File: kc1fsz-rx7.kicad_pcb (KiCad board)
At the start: 2 copper layers, 35.8 x 29.5 mm, 18 parts, among them J1 IQ, J2 Power, J3 Config, J4 Conn_01x06, U1 PCM1804DBR

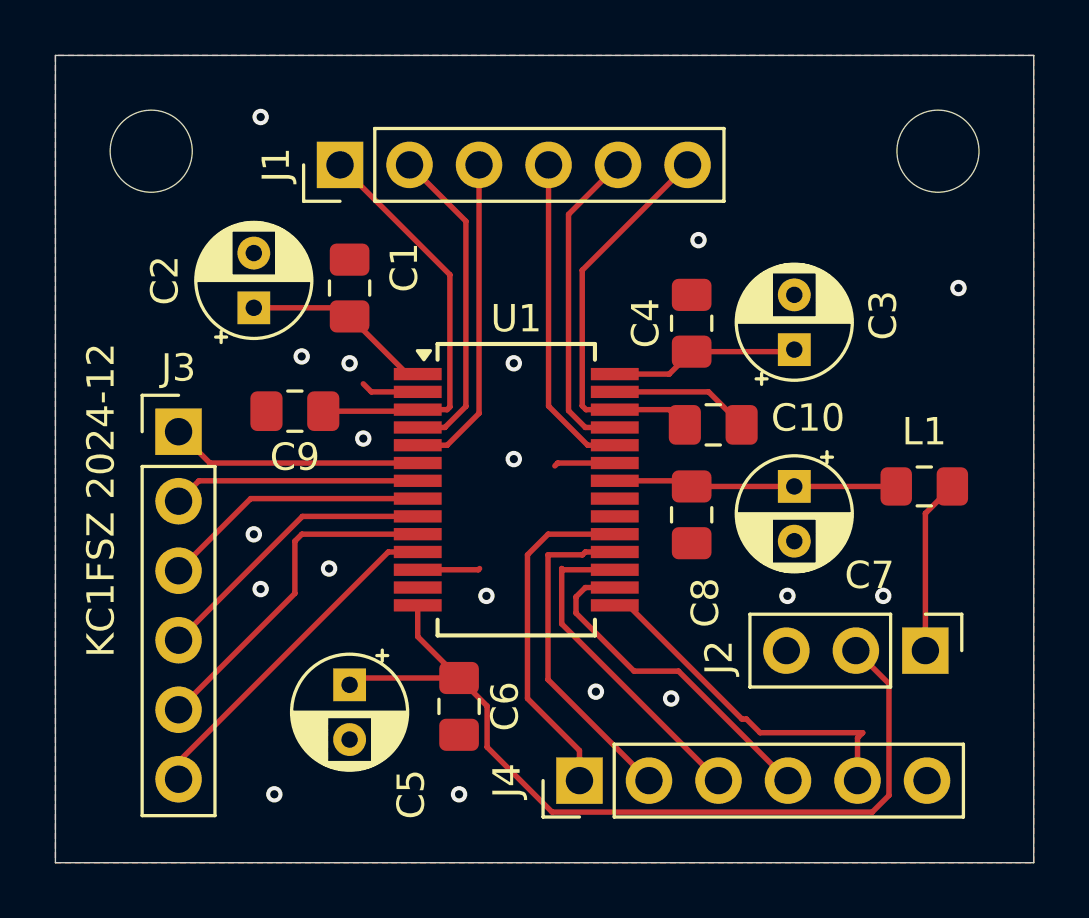
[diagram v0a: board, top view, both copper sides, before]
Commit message: Final board being sent to OSHPARK
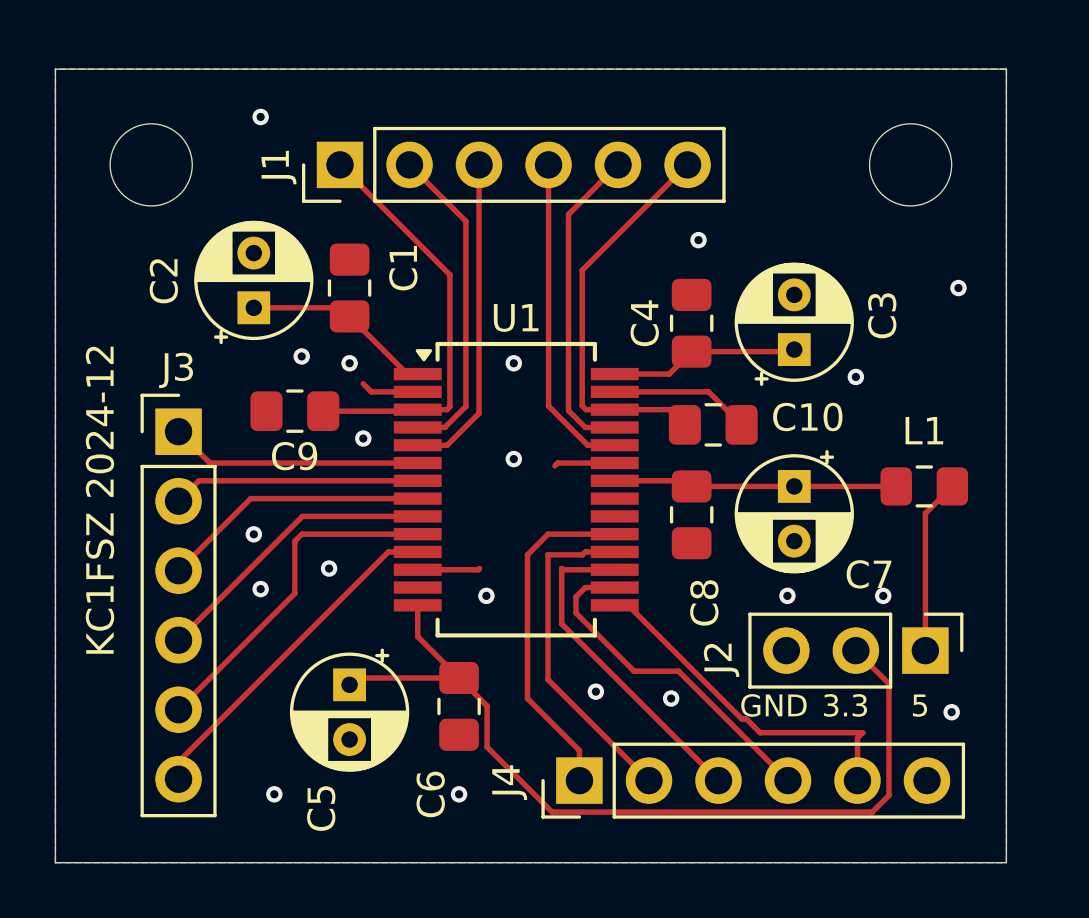
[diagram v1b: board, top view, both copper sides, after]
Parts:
- moved H2 1.12 mm to (174.0, 99.5)
- moved H1 0.50 mm to (146.2, 99.5)
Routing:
- net GND: vias 18 -> 20
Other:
- board size 35.8 x 29.5 mm -> 34.8 x 29 mm
- board text added: "3.3"
- board text added: "5"
- board text added: "GND"
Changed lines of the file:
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@@
 		(legacy_teardrops no)
 	)
-	(paper "A4")
+	(paper "USLetter")
+	(title_block
+		(title "PCM1804 Breakout Board")
+		(date "2024-12-03")
+		(rev "1")
+		(company "Bruce MacKinnon KC1FSZ")
+	)
 	(layers
 		(0 "F.Cu" signal)
@@
 			(sketchpadsonfab no)
 			(subtractmaskfromsilk no)
-			(outputformat 1)
+			(outputformat 4)
 			(mirror no)
-			(drillshape 1)
+			(drillshape 0)
 			(scaleselection 1)
-			(outputdirectory "")
+			(outputdirectory "docs")
 		)
 	)
@@
 		(tags "capacitor handsolder")
 		(property "Reference" "C6"
-			(at 0 -1.68 90)
+			(at 3.2125 1 90)
 			(layer "F.SilkS")
 			(effects
@@
 	(footprint "MountingHole:MountingHole_3mm"
 		(layer "F.Cu")
-		(at 175 99)
+		(at 174 99.5)
 		(descr "Mounting Hole 3mm, no annular")
 		(tags "mounting hole 3mm no annular")
@@
 		(tags "CP Radial series Radial pin pitch 2.00mm  diameter 4mm Electrolytic Capacitor")
 		(property "Reference" "C5"
-			(at 4 -2.25 90)
+			(at 4.5 1 90)
 			(layer "F.SilkS")
 			(effects
@@
 	(footprint "MountingHole:MountingHole_3mm"
 		(layer "F.Cu")
-		(at 146.25 99)
+		(at 146.25 99.5)
 		(descr "Mounting Hole 3mm, no annular")
 		(tags "mounting hole 3mm no annular")
@@
 	)
 	(gr_rect
-		(start 142.75 95.5)
-		(end 178.5 125)
+		(start 142.75 96)
+		(end 177.5 125)
 		(stroke
 			(width 0.05)
@@
 		)
 	)
+	(gr_text "GND"
+		(at 167.75 119.75 0)
+		(layer "F.SilkS")
+		(effects
+			(font
+				(size 0.8 0.8)
+				(thickness 0.1)
+			)
+			(justify left bottom)
+		)
+	)
+	(gr_text "3.3"
+		(at 170.75 119.75 0)
+		(layer "F.SilkS")
+		(effects
+			(font
+				(size 0.8 0.8)
+				(thickness 0.1)
+			)
+			(justify left bottom)
+		)
+	)
+	(gr_text "5"
+		(at 174 119.75 0)
+		(layer "F.SilkS")
+		(effects
+			(font
+				(size 0.8 0.8)
+				(thickness 0.1)
+			)
+			(justify left bottom)
+		)
+	)
 	(segment
 		(start 155.99 107.145)
@@
 	)
 	(via
+		(at 172 107.25)
+		(size 0.6)
+		(drill 0.3)
+		(layers "F.Cu" "B.Cu")
+		(free yes)
+		(net 2)
+	)
+	(via
 		(at 150.25 115)
 		(size 0.6)
@@
 	)
 	(via
+		(at 175.5 119.5)
+		(size 0.6)
+		(drill 0.3)
+		(layers "F.Cu" "B.Cu")
+		(free yes)
+		(net 2)
+	)
+	(via
 		(at 150.25 97.75)
 		(size 0.6)
@@
 		(polygon
 			(pts
-				(xy 142.75 95.5) (xy 142.75 125) (xy 178.5 125) (xy 178.5 95.5)
+				(xy 142.75 96) (xy 142.75 125) (xy 177.5 125) (xy 177.5 96)
 			)
 		)
@@
 		(polygon
 			(pts
-				(xy 142.75 95.5) (xy 142.75 125) (xy 178.5 125) (xy 178.5 95.5)
+				(xy 142.75 96) (xy 142.75 125) (xy 177.5 125) (xy 177.5 96)
 			)
 		)
